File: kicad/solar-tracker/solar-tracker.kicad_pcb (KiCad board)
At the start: 2 copper layers, 160.5 x 72.5 mm, 17 parts, among them J1 Barrel_Jack_Switch, J2 Conn_01x08_Pin, J3 Conn_01x08_Pin, M1 Motor_Servo, M2 Motor_Servo

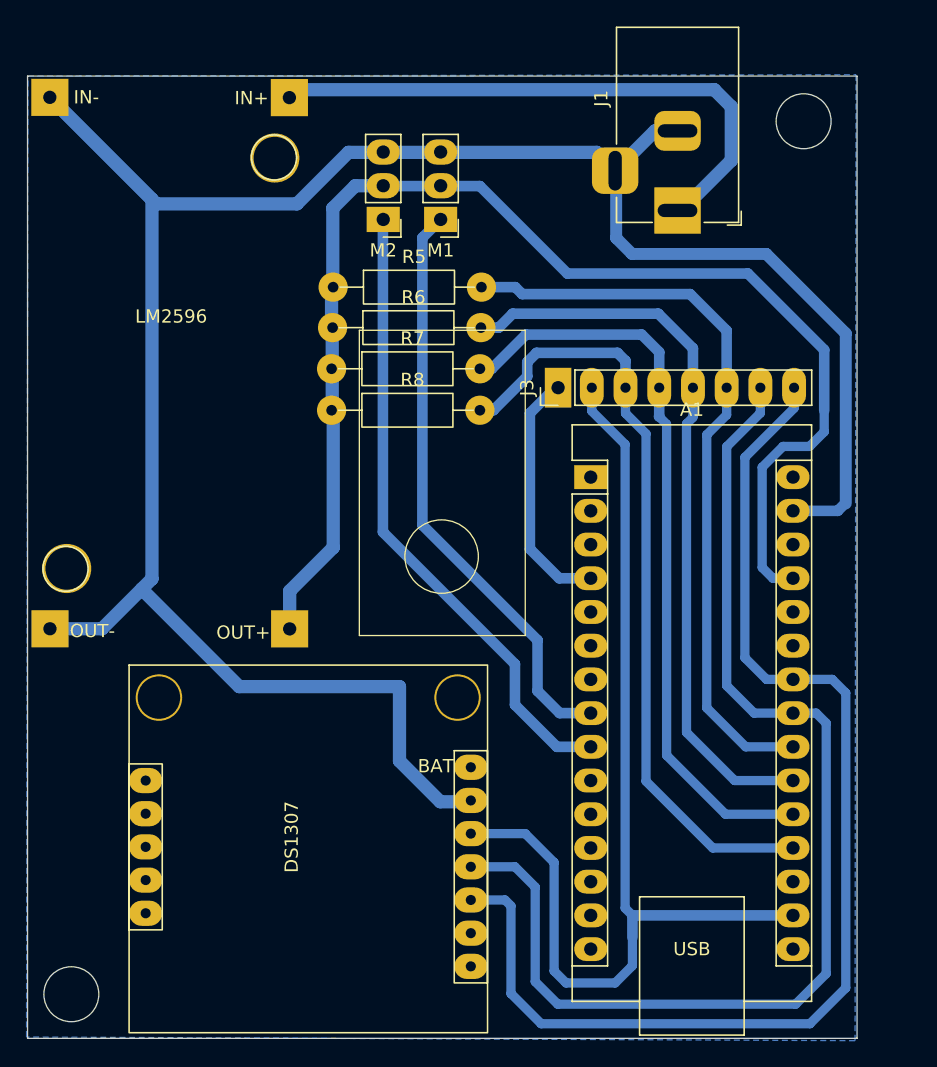
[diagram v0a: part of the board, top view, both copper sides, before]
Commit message: update
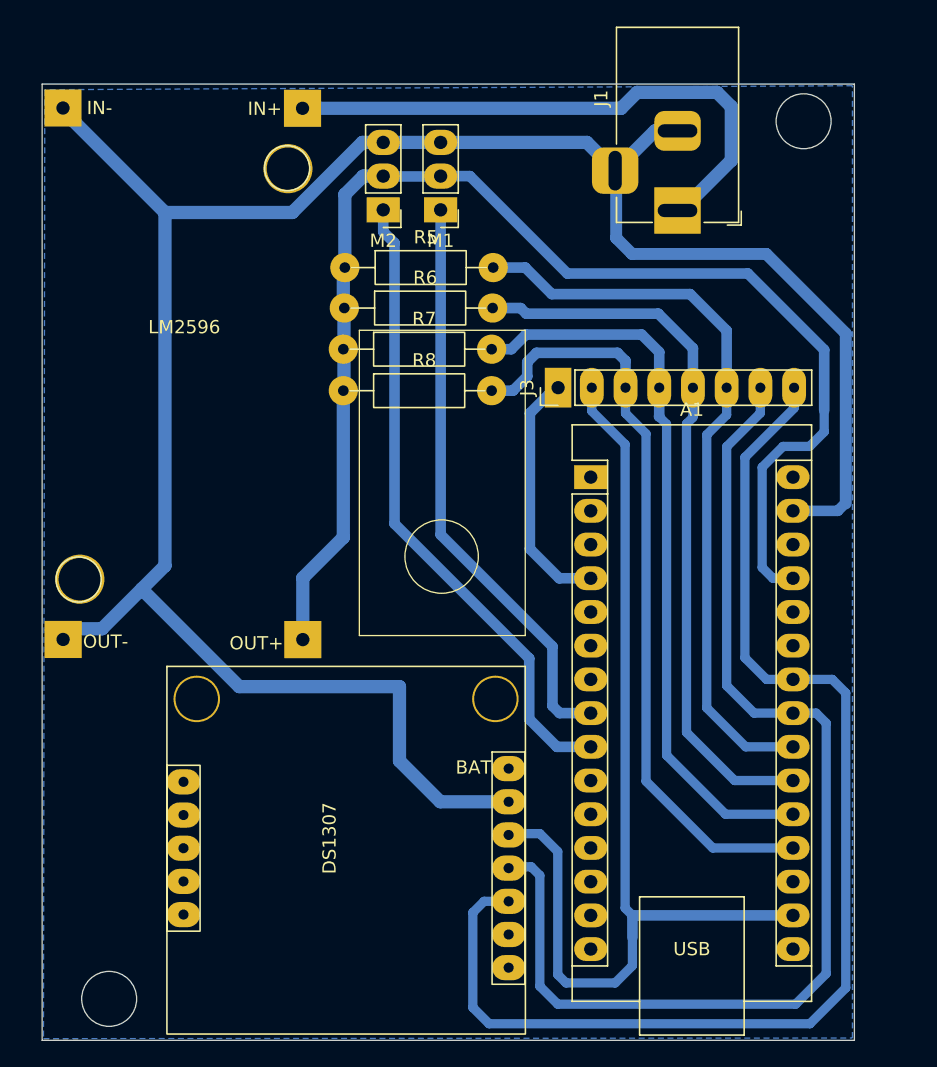
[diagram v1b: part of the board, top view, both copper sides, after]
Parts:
- moved DS1307 2.85 mm to (38.9, 108.2)
- moved R6 1.72 mm to (58.1, 53.5)
- moved R7 1.72 mm to (58.0, 56.6)
- moved R8 1.72 mm to (58.0, 59.7)
- moved R5 1.72 mm to (58.1, 50.5)
- moved LM2596 1.28 mm to (29.6, 80.0)
- moved M1 0.73 mm to (59.5, 46.1)
- moved M2 0.73 mm to (55.2, 46.1)
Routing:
- net GND: track 294.2 -> 284.8 mm
- net /Placa_sensor/SCL: track 120.1 -> 123.0 mm
- net +3V3: track 110.2 -> 108.0 mm
- net /Placa_sensor/SDA: track 117.6 -> 115.5 mm
- net /Placa_sensor/LDR2: track 121.3 -> 119.8 mm
- net /Placa_sensor/LDR1: track 88.9 -> 87.4 mm
- net /Placa_sensor/LDR3: track 61.5 -> 60.4 mm
- net +5V: track 98.3 -> 99.3 mm
- net Net-(LM2596-IN-): track 43.7 -> 42.9 mm
- net Net-(A1-D6): track 47.7 -> 48.4 mm
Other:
- board size 160.5 x 72.5 mm -> 159.4 x 72 mm
